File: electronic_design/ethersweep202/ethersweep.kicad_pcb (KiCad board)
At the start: 2 copper layers, 79 x 38 mm, 73 parts, among them J1 AVR-ISP-6, J2 Conn_01x02_Male, J3 Conn_01x04_Female, J4 Conn_01x02_Male, J5 Conn_01x02_Male, J6 HR911105A, J7 Conn_01x06_Female, J8 AVR-ISP-6, J9 Conn_01x06_Male, M1 Stepper_Motor_bipolar, SW1 SW_Push, U1 ENC28J60x-SS, U2 ATmega328-AU, U3 DRV8825PWPR, U4 AMS1117-3.3, U5 AS5600, Y1 Crystal_25MHz, Y3 Crystal

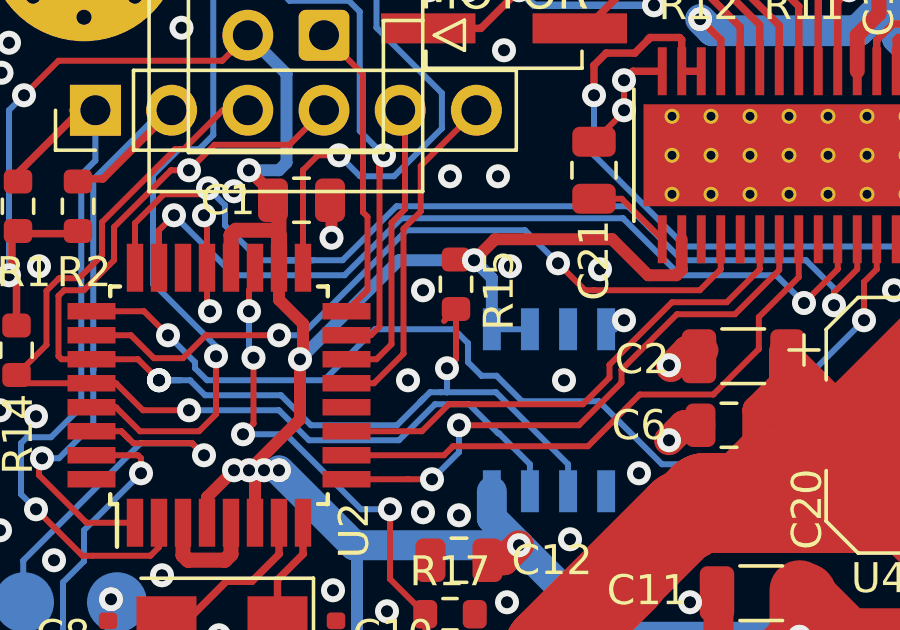
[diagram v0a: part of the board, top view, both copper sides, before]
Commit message: minor v202 changes
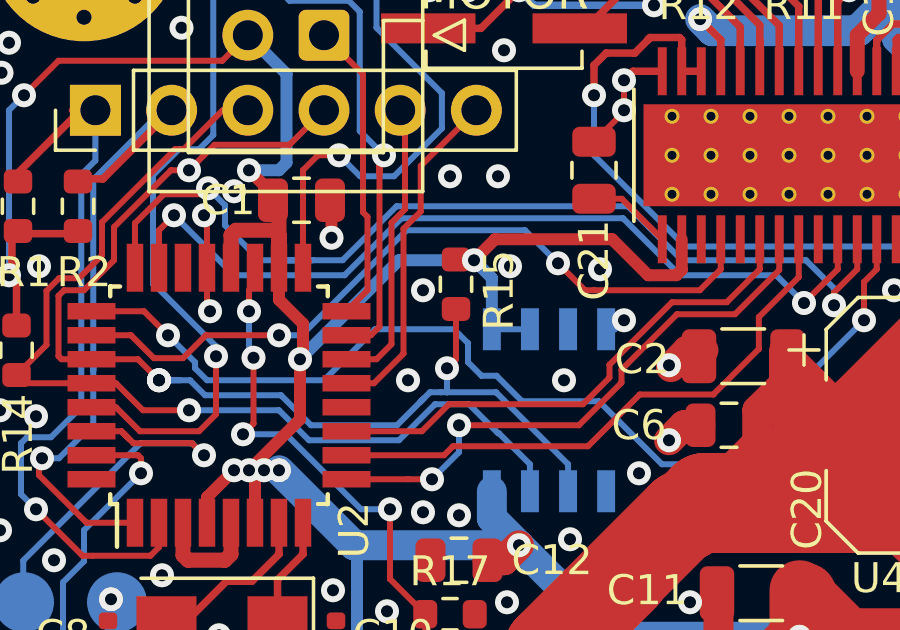
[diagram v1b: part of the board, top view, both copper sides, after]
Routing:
- net SDA: track 78.2 -> 77.6 mm
